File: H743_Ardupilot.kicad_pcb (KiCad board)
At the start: 2 copper layers, 36.5 x 36.5 mm, 148 parts, among them J1 Conn_01x04, J10 Conn_01x03, J11 Conn_01x03, J12 10067099-200LF, J2 Conn_01x04, J3 Conn_01x04, J4 Conn_01x06, J5 Conn_01x04, J6 Conn_01x04, J7 Conn_01x04, J8 Conn_01x04, J9 Conn_01x04, Q1 AO3400A, U1 USBLC6-2P6, U10 LSM6DSV16X, U12 BMP581, U14 ZX-SH1.0-8PWT, U2 STM32H743VIT6, U3 LMR43620R5RPER, U4 LMR604303SRAKRQ1, U5 AP7361C-33FGE-7, U6 AP7361C-33FGE-7, U8 ZX-SH1.0-4PWT, U9 BMI088

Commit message: Sync U1 PCB footprint name with source CAD
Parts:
- U1: footprint H743_Custom:ST_USBLC6-2P6_SOT-666 -> H743_Custom:SOT50P160X60-6N
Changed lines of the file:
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@@
 		)
 	)
-	(footprint "H743_Custom:ST_USBLC6-2P6_SOT-666"
+	(footprint "H743_Custom:SOT50P160X60-6N"
 		(layer "F.Cu")
 		(at 82.5 88 -90)

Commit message: Sync U1 and D2 dedicated footprint library names on PCB
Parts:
- D2: footprint H743_Custom:SMAJ30CA_SMA_LTF -> SMAJ30CA:SMASeries_LTF
- U1: footprint H743_Custom:SOT50P160X60-6N -> USBLC6_2P6:SOT50P160X60-6N
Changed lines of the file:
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@@
 		)
 	)
-	(footprint "H743_Custom:SMAJ30CA_SMA_LTF"
+	(footprint "SMAJ30CA:SMASeries_LTF"
 		(layer "F.Cu")
 		(at 83.5 93 180)
@@
 		)
 	)
-	(footprint "H743_Custom:SOT50P160X60-6N"
+	(footprint "USBLC6_2P6:SOT50P160X60-6N"
 		(layer "F.Cu")
 		(at 82.5 88 -90)

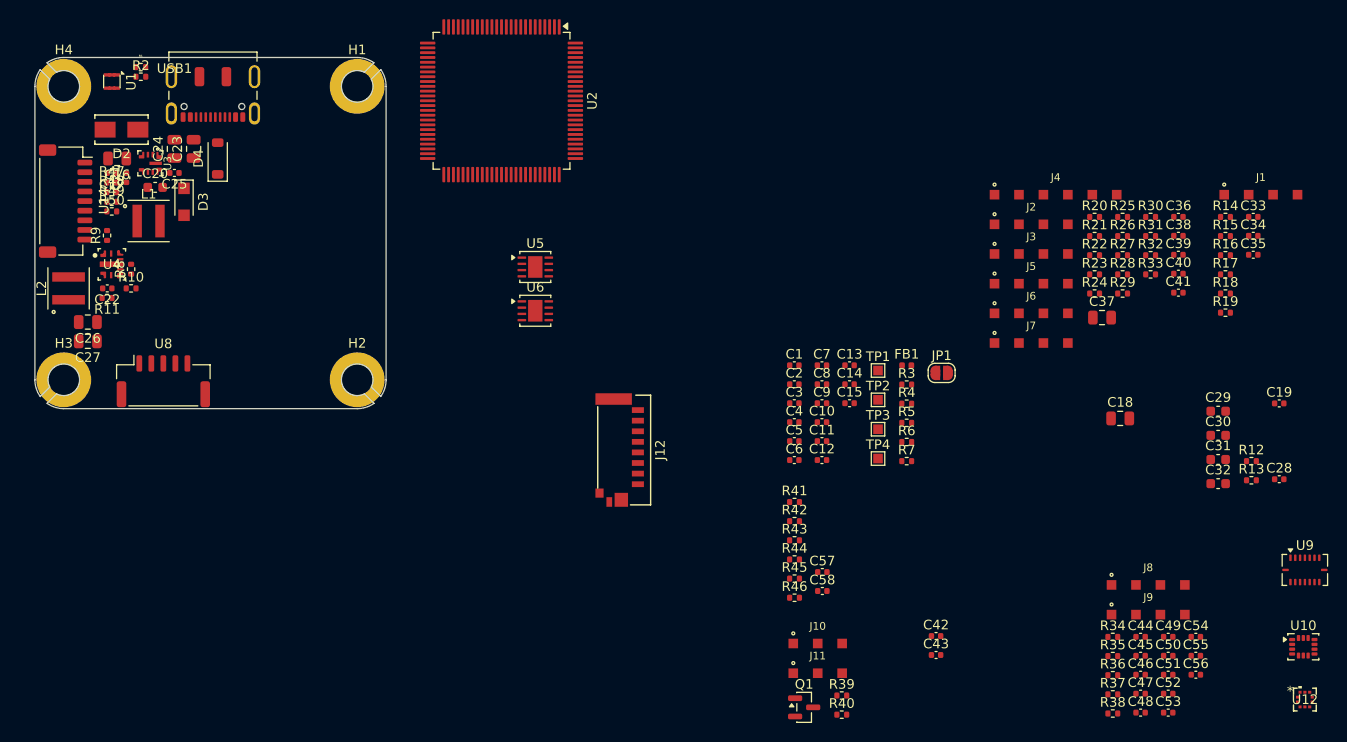
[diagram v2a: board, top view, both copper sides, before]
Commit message: update pcb
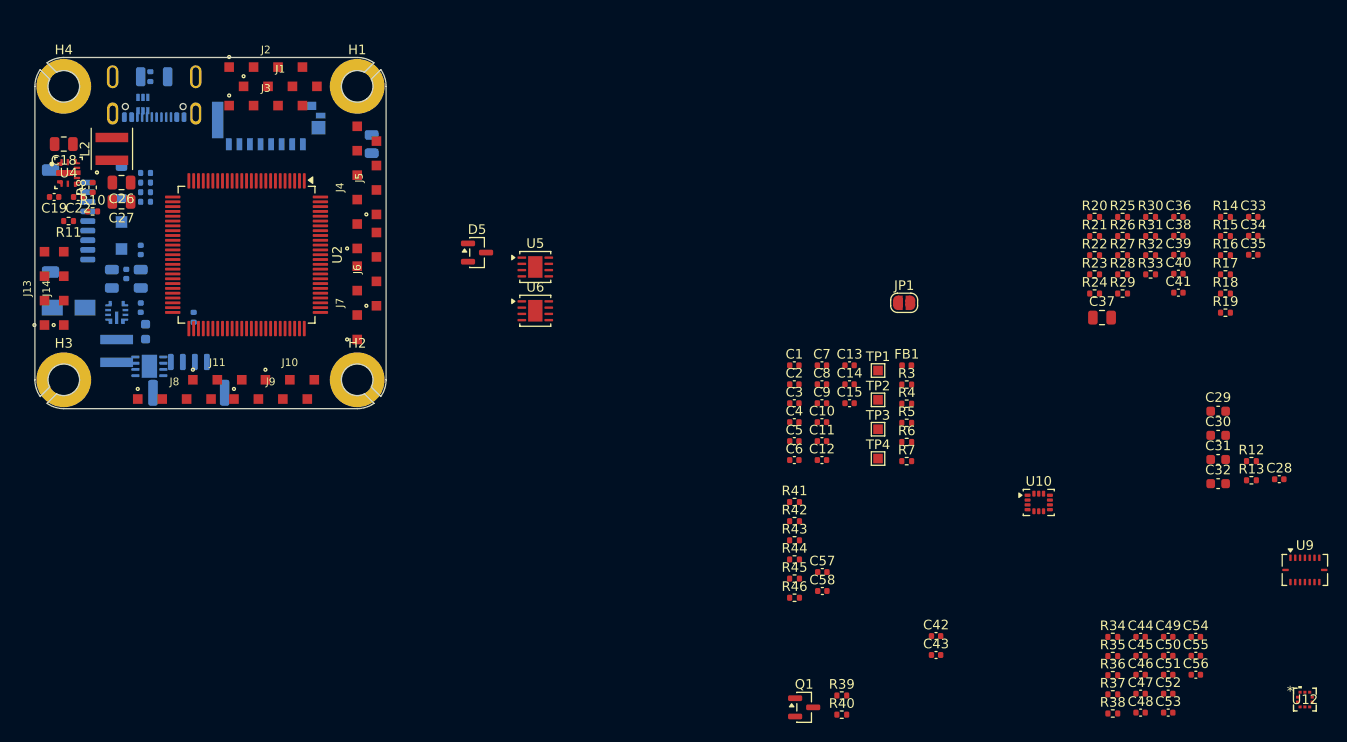
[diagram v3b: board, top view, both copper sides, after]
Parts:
- added D5: PESD2CAN, Package_TO_SOT_SMD:SOT-23, F.Cu at (120.5, 105.8)
- added J13: Can1_2, H743_Custom:SolderPadArray_1x04_P2.54mm_1x1mm, F.Cu at (75.5, 109.5)
- added J14: Can1_1, H743_Custom:SolderPadArray_1x04_P2.54mm_1x1mm, F.Cu at (77.5, 109.5)
- added U7: TJA1051TK/3,118, Package_SON:HVSON-8-1EP_3x3mm_P0.65mm_EP1.6x2.4mm, B.Cu at (86.4, 117.6)
- C16, C17, C20, C21, C23, C24, C25, D2, D3, D4, J12, L1, R1, R2, R47, R48, R49, R50, R9, U1, U3, USB1: moved to B.Cu
- J1: value Conn_01x04 -> Analog
- J10: value Conn_01x03 -> Led ext
- J11: value Conn_01x03 -> Buzzer
- J2: value Conn_01x04 -> Uart1
- J3: value Conn_01x04 -> Uart4
- J4: value Conn_01x06 -> Uart7
- J5: value Conn_01x04 -> Uart(
- J6: value Conn_01x04 -> Uart6
- J7: value Conn_01x04 -> Uart3
- J8: value Conn_01x04 -> I2C1
- J9: value Conn_01x04 -> I2C_2
- U14: value ZX-SH1.0-8PWT -> SM08B-SRSS-TB(LF)(SN); moved to B.Cu
- U8: value ZX-SH1.0-4PWT -> SM04B-GHS-TB(LF)(SN); footprint Connector_JST:JST_GH_SM05B-GHS-TB_1x05-1MP_P1.25mm_Horizontal -> H743_Custom:JST_GH_SM04B-GHS-TB_1x04_P1.25mm_Horizontal_GNDtabs; moved to B.Cu
- moved C19 129.1 mm to (76.5, 100.0), turned to 180 degrees
- moved C18 113.4 mm to (77.5, 94.5), turned to 180 degrees
- moved J8 103.0 mm to (89.0, 121.0)
- moved J1 102.5 mm to (100.0, 88.5)
- moved J9 93.9 mm to (99.0, 121.0)
- moved J2 81.2 mm to (98.5, 86.5)
- moved J3 81.0 mm to (98.5, 90.5)
- moved J4 72.6 mm to (108.0, 99.0), turned to 90 degrees
- moved J7 70.2 mm to (108.0, 111.0), turned to 90 degrees
- moved J11 69.5 mm to (93.5, 119.0)
- moved J5 68.9 mm to (110.0, 98.0), turned to 90 degrees
- moved J6 68.2 mm to (110.0, 107.5), turned to 90 degrees
- moved J10 61.3 mm to (101.0, 119.0)
- moved J12 50.1 mm to (98.5, 95.8), turned to 0 degrees
- moved U10 31.3 mm to (178.8, 131.8)
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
